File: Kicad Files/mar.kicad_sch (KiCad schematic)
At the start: 37 parts, among them U10 74LS173, U11 74LS173, U12 74LS173, U9 74LS173

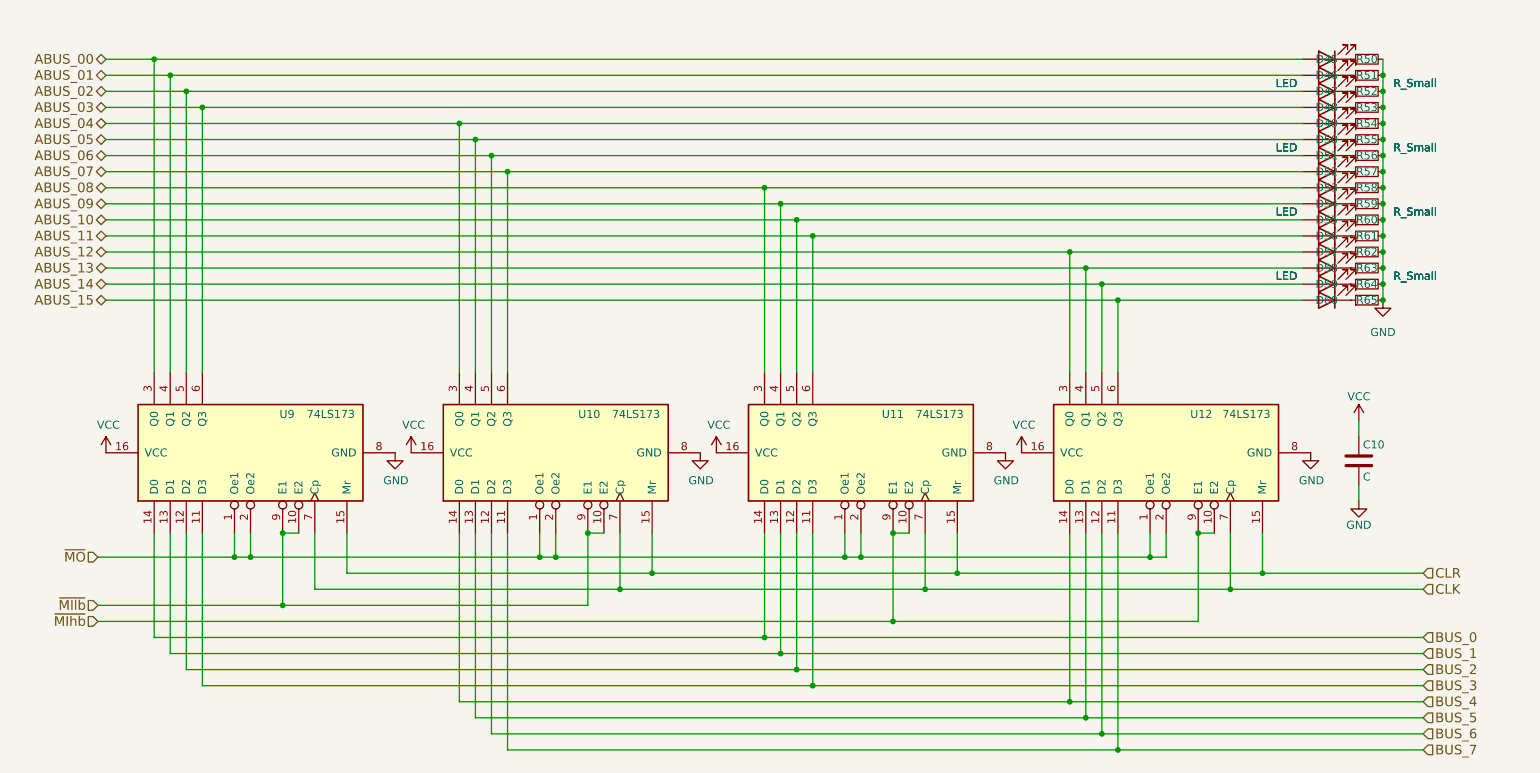
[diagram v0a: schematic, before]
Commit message: im sooo stupiiid
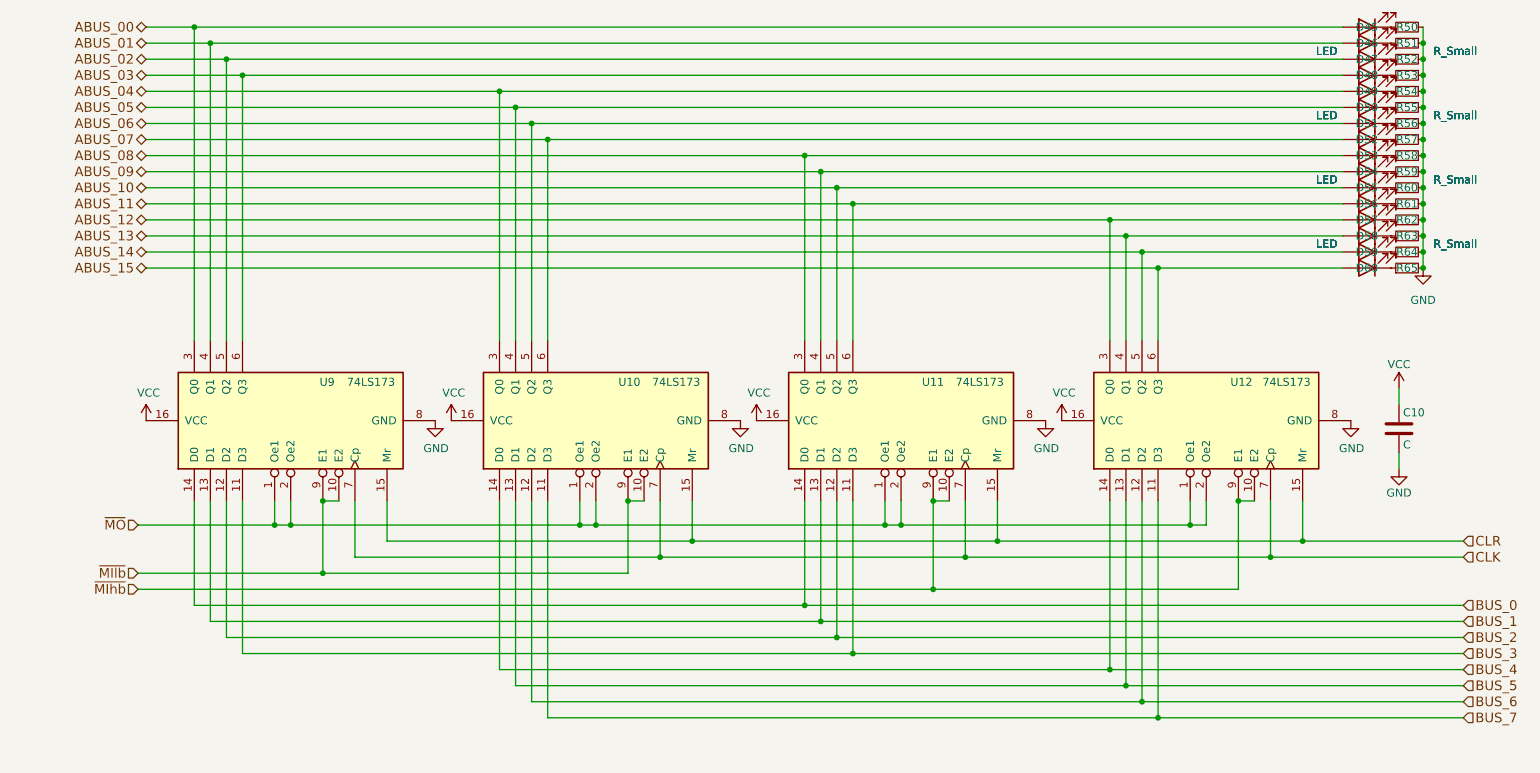
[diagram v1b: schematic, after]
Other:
- moved on the sheet: C10, D45, D46, D47, D48, D49, D50, D51, D52, D53, D54, D55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
